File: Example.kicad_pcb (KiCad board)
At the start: 2 copper layers, 30 x 30 mm, 5 parts, among them J1 Conn_01x02, SW1 SW_Push

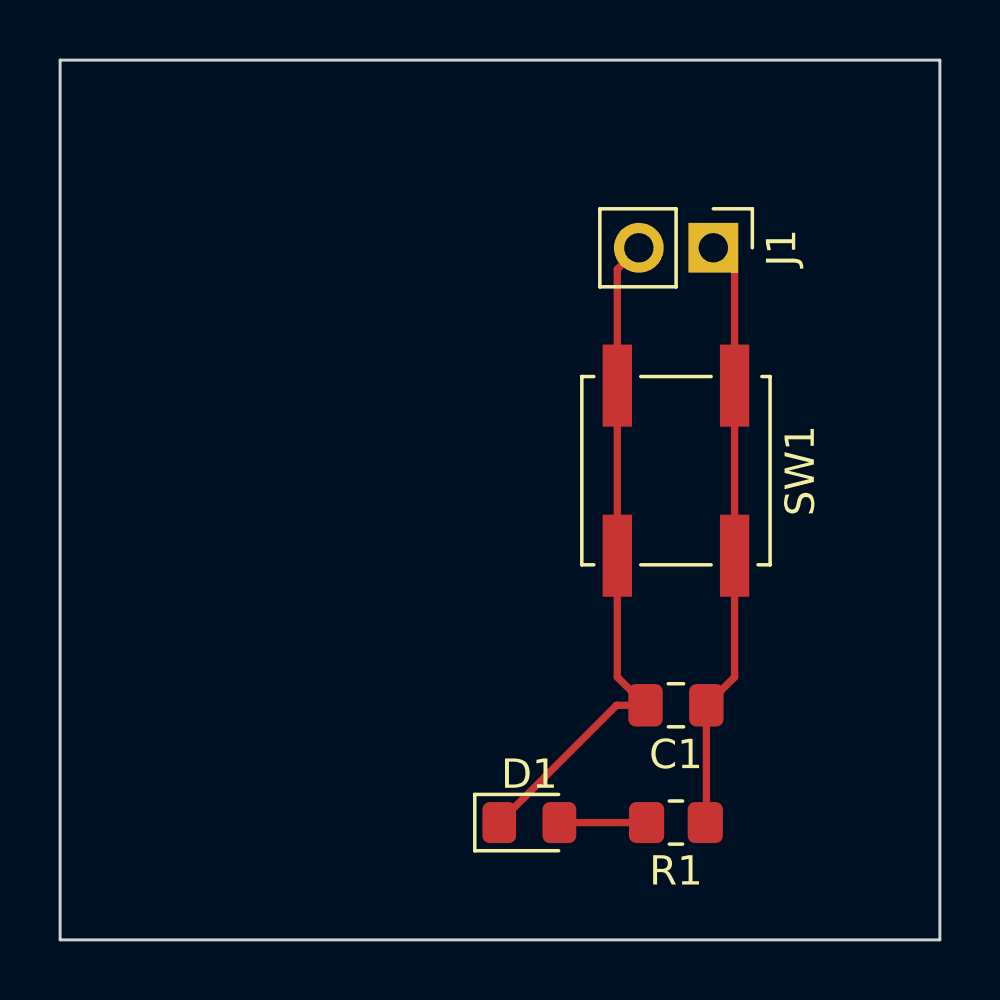
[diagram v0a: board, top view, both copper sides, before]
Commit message: <minor> Add cleanup and teardrop ex
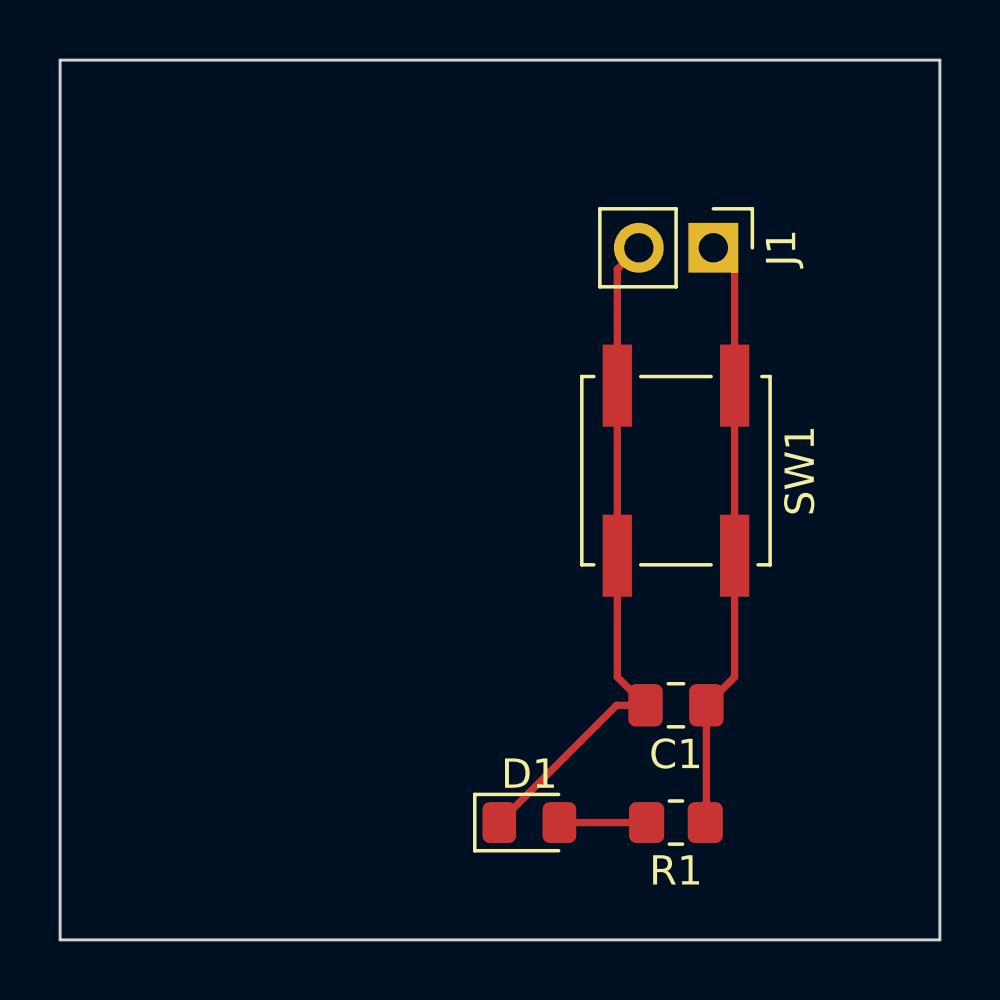
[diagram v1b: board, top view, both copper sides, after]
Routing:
- net +5V: track 20.3 -> 19.2 mm
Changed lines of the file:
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@@
   (gr_rect locked (start 0 0) (end 30 30)
     (stroke (width 0.1) (type default)) (fill none) (layer "Edge.Cuts"))
-  (segment (start 22.0375 25.9625) (end 22 26) (width 0.25) (layer "F.Cu") (net 1))
   (segment (start 22.0375 22) (end 22.0375 25.9625) (width 0.25) (layer "F.Cu") (net 1))
   (segment (start 23 21.0375) (end 23 16.9) (width 0.25) (layer "F.Cu") (net 1))
   (segment (start 23 11.1) (end 23 7.125) (width 0.25) (layer "F.Cu") (net 1))
   (segment (start 23 11.1) (end 23 16.9) (width 0.25) (layer "F.Cu") (net 1))
-  (segment (start 23 7.125) (end 22.275 6.4) (width 0.25) (layer "F.Cu") (net 1))
   (segment (start 22.0375 22) (end 23 21.0375) (width 0.25) (layer "F.Cu") (net 1))
   (segment (start 18.975 22) (end 14.975 26) (width 0.25) (layer "F.Cu") (net 2))
@@
   (segment (start 19.9625 22) (end 18.975 22) (width 0.25) (layer "F.Cu") (net 2))
   (segment (start 20 26) (end 17.025 26) (width 0.25) (layer "F.Cu") (net 3))
+  (zone (net 1) (net_name "+5V") (layer "F.Cu") (name "$teardrop_padvia$") (hatch edge 0.5)
+    (priority 30001)
+    (attr (teardrop (type padvia)))
+    (connect_pads yes (clearance 0))
+    (min_thickness 0.0254) (filled_areas_thickness no)
+    (fill yes (thermal_gap 0.5) (thermal_bridge_width 0.5) (island_removal_mode 1) (island_area_min 10))
+    (polygon
+      (pts
+        (xy 23.125 9.2)
+        (xy 22.875 9.2)
+        (xy 22.5 9.7)
+        (xy 23 11.101)
+        (xy 23.5 9.7)
+      )
+    )
+  )
+  (zone (net 3) (net_name "Net-(D1-A)") (layer "F.Cu") (name "$teardrop_padvia$") (hatch edge 0.5)
+    (priority 30007)
+    (attr (teardrop (type padvia)))
+    (connect_pads yes (clearance 0))
+    (min_thickness 0.0254) (filled_areas_thickness no)
+    (fill yes (thermal_gap 0.5) (thermal_bridge_width 0.5) (island_removal_mode 1) (island_area_min 10))
+    (polygon
+      (pts
+        (xy 18.8 25.875)
+        (xy 18.8 26.125)
+        (xy 19.455331 26.6)
+        (xy 20.001 26)
+        (xy 19.455331 25.4)
+      )
+    )
+  )
+  (zone (net 3) (net_name "Net-(D1-A)") (layer "F.Cu") (name "$teardrop_padvia$") (hatch edge 0.5)
+    (priority 30008)
+    (attr (teardrop (type padvia)))
+    (connect_pads yes (clearance 0))
+    (min_thickness 0.0254) (filled_areas_thickness no)
+    (fill yes (thermal_gap 0.5) (thermal_bridge_width 0.5) (island_removal_mode 1) (island_area_min 10))
+    (polygon
+      (pts
+        (xy 18.175 26.125)
+        (xy 18.175 25.875)
+        (xy 17.561373 25.425)
+        (xy 17.024 26)
+        (xy 17.561373 26.575)
+      )
+    )
+  )
+  (zone (net 1) (net_name "+5V") (layer "F.Cu") (name "$teardrop_padvia$") (hatch edge 0.5)
+    (priority 30003)
+    (attr (teardrop (type padvia)))
+    (connect_pads yes (clearance 0))
+    (min_thickness 0.0254) (filled_areas_thickness no)
+    (fill yes (thermal_gap 0.5) (thermal_bridge_width 0.5) (island_removal_mode 1) (island_area_min 10))
+    (polygon
+      (pts
+        (xy 22.875 13)
+        (xy 23.125 13)
+        (xy 23.5 12.5)
+        (xy 23 11.099)
+        (xy 22.5 12.5)
+      )
+    )
+  )
+  (zone (net 1) (net_name "+5V") (layer "F.Cu") (name "$teardrop_padvia$") (hatch edge 0.5)
+    (priority 30002)
+    (attr (teardrop (type padvia)))
+    (connect_pads yes (clearance 0))
+    (min_thickness 0.0254) (filled_areas_thickness no)
+    (fill yes (thermal_gap 0.5) (thermal_bridge_width 0.5) (island_removal_mode 1) (island_area_min 10))
+    (polygon
+      (pts
+        (xy 23.125 15)
+        (xy 22.875 15)
+        (xy 22.5 15.5)
+        (xy 23 16.901)
+        (xy 23.5 15.5)
+      )
+    )
+  )
+  (zone (net 1) (net_name "+5V") (layer "F.Cu") (name "$teardrop_padvia$") (hatch edge 0.5)
+    (priority 30000)
+    (attr (teardrop (type padvia)))
+    (connect_pads yes (clearance 0))
+    (min_thickness 0.0254) (filled_areas_thickness no)
+    (fill yes (thermal_gap 0.5) (thermal_bridge_width 0.5) (island_removal_mode 1) (island_area_min 10))
+    (polygon
+      (pts
+        (xy 22.875 18.8)
+        (xy 23.125 18.8)
+        (xy 23.5 18.3)
+        (xy 23 16.899)
+        (xy 22.5 18.3)
+      )
+    )
+  )
+  (zone (net 1) (net_name "+5V") (layer "F.Cu") (name "$teardrop_padvia$") (hatch edge 0.5)
+    (priority 30005)
+    (attr (teardrop (type padvia)))
+    (connect_pads yes (clearance 0))
+    (min_thickness 0.0254) (filled_areas_thickness no)
+    (fill yes (thermal_gap 0.5) (thermal_bridge_width 0.5) (island_removal_mode 1) (island_area_min 10))
+    (polygon
+      (pts
+        (xy 22.1625 24.7)
+        (xy 21.9125 24.7)
+        (xy 21.41903 25.454329)
+        (xy 22 26.001)
+        (xy 22.58097 25.454329)
+      )
+    )
+  )
+  (zone (net 1) (net_name "+5V") (layer "F.Cu") (name "$teardrop_padvia$") (hatch edge 0.5)
+    (priority 30004)
+    (attr (teardrop (type padvia)))
+    (connect_pads yes (clearance 0))
+    (min_thickness 0.0254) (filled_areas_thickness no)
+    (fill yes (thermal_gap 0.5) (thermal_bridge_width 0.5) (island_removal_mode 1) (island_area_min 10))
+    (polygon
+      (pts
+        (xy 23.125 21.006726)
+        (xy 22.875 21.006726)
+        (xy 21.922617 21.275)
+        (xy 22.0375 22.001)
+        (xy 22.625 22.238781)
+      )
+    )
+  )
+  (zone (net 1) (net_name "+5V") (layer "F.Cu") (name "$teardrop_padvia$") (hatch edge 0.5)
+    (priority 30006)
+    (attr (teardrop (type padvia)))
+    (connect_pads yes (clearance 0))
+    (min_thickness 0.0254) (filled_areas_thickness no)
+    (fill yes (thermal_gap 0.5) (thermal_bridge_width 0.5) (island_removal_mode 1) (island_area_min 10))
+    (polygon
+      (pts
+        (xy 21.9125 23.3125)
+        (xy 22.1625 23.3125)
+        (xy 22.60597 22.570671)
+        (xy 22.0375 21.999)
+        (xy 21.46903 22.570671)
+      )
+    )
+  )
   (zone (net 2) (net_name "GND") (layers "F&B.Cu") (hatch edge 0.25)
     (connect_pads (clearance 0.25))
